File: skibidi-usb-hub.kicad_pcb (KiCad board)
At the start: 4 copper layers, 70 x 70 mm, 99 parts, among them SW1 B3U-1100PM, SW2 B3U-1100PM, T1 H1102NLT_C20623173, T2 H1102NLT_C20623173, U1 CH334F_C5187527, U10 PJ-320A-4P DIP, U2 CH217K, U3 GT-USB-7010ASV, U4 GT-USB-7010ASV, U5 RTL8152B-VB-CG, U6 GT-USB-7010ASV, U7 RTL8152B-VB-CG, U8 CH334F_C5187527, U9 HS-100B, X1 X322516MLB4SI, X2 X322516MLB4SI

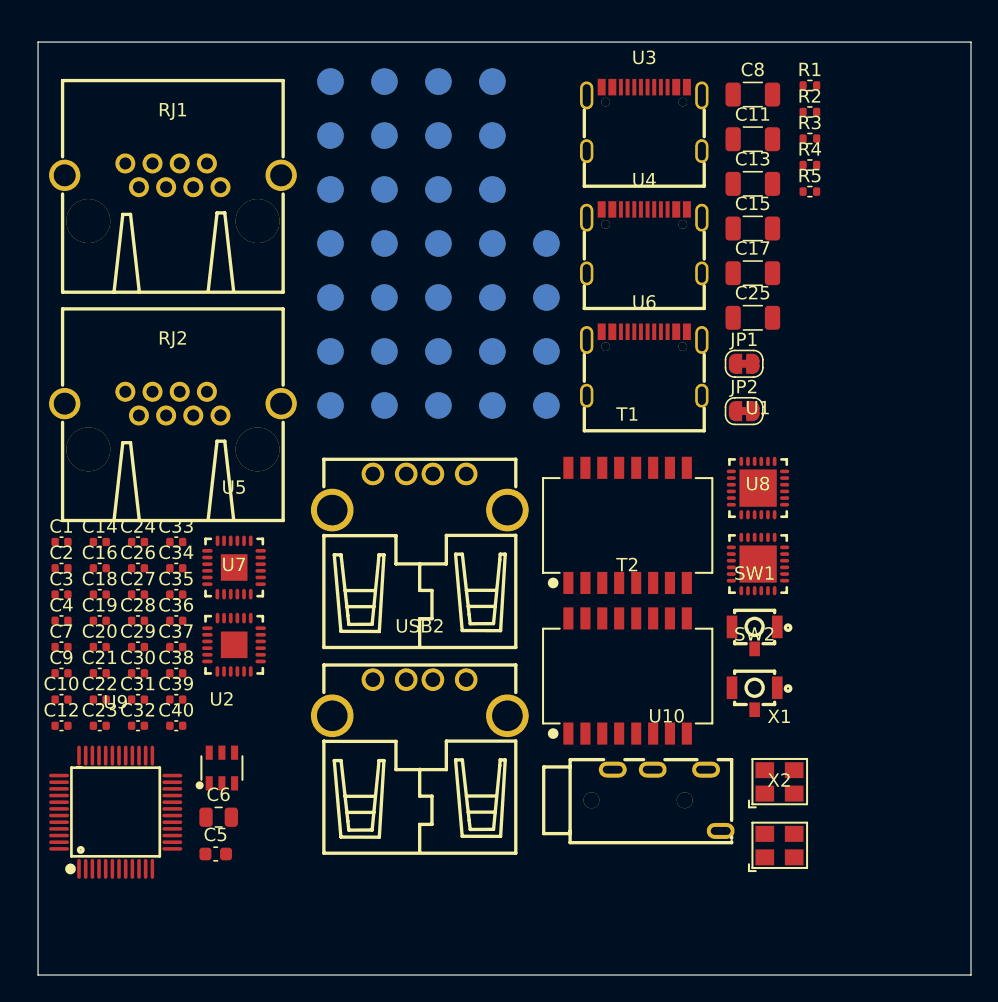
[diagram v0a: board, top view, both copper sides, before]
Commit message: PCB done!!!
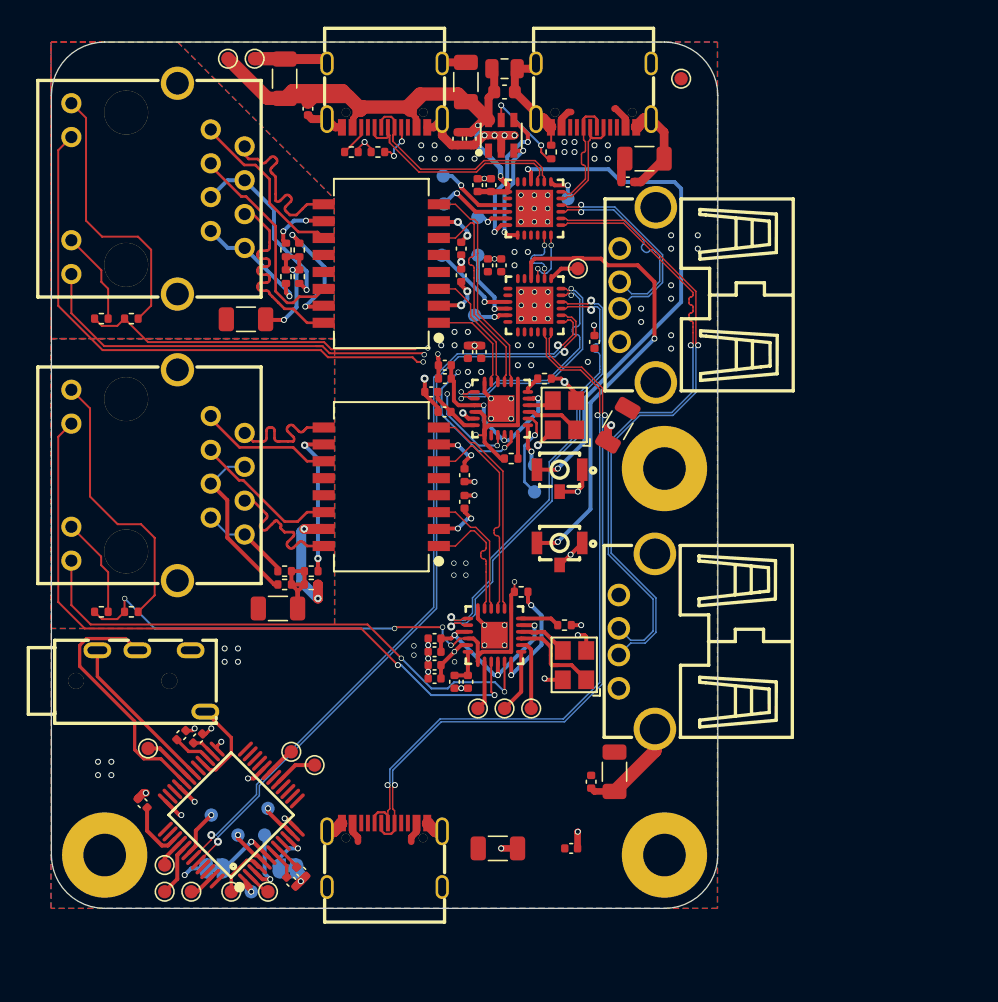
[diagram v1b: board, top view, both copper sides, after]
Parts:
- removed TP10, TP27, TP9: TestPoint, TestPoint:TestPoint_Pad_D2.0mm
- added C41: 1n, Capacitor_SMD:C_1206_3216Metric, F.Cu at (135.6, 80.8)
- added C42: 1n, Capacitor_SMD:C_1206_3216Metric, F.Cu at (138.0, 102.5)
- added H1: MountingHole, MountingHole:MountingHole_3.2mm_M3_Pad, F.Cu at (167.0, 121.0)
- added H2: MountingHole, MountingHole:MountingHole_3.2mm_M3_Pad, F.Cu at (167.0, 92.0)
- added H3: MountingHole, MountingHole:MountingHole_3.2mm_M3_Pad, F.Cu at (125.0, 121.0)
- added R10: 75, Resistor_SMD:R_0402_1005Metric, F.Cu at (139.6, 77.6)
- added R11: 75, Resistor_SMD:R_0402_1005Metric, F.Cu at (138.6, 77.6)
- added R12: 75, Resistor_SMD:R_0402_1005Metric, F.Cu at (140.5, 100.7)
- added R13: 75, Resistor_SMD:R_0402_1005Metric, F.Cu at (140.5, 99.7)
- added R14: 75, Resistor_SMD:R_0402_1005Metric, F.Cu at (138.5, 100.7)
- added R15: 75, Resistor_SMD:R_0402_1005Metric, F.Cu at (138.5, 99.7)
- added R16: 470, Resistor_SMD:R_0402_1005Metric, F.Cu at (127.0, 80.8)
- added R17: 470, Resistor_SMD:R_0402_1005Metric, F.Cu at (124.8, 80.8)
- added R18: 470, Resistor_SMD:R_0402_1005Metric, F.Cu at (127.0, 102.8)
- added R19: 470, Resistor_SMD:R_0402_1005Metric, F.Cu at (124.8, 102.8)
- added R6: 5.1k, Resistor_SMD:R_0402_1005Metric, F.Cu at (145.5, 68.2)
- added R7: 5.1k, Resistor_SMD:R_0402_1005Metric, F.Cu at (143.5, 68.2)
- added R8: 75, Resistor_SMD:R_0402_1005Metric, F.Cu at (139.6, 75.6)
- added R9: 75, Resistor_SMD:R_0402_1005Metric, F.Cu at (138.6, 75.6)
- JP1, JP2: moved to B.Cu
- RJ1, RJ2: value X12ADGWA3DY1027 -> R-RJ45S08P-C000; footprint easyeda2kicad:RJ45-TH_XKB_X12ADHWA3DY1027 -> easyeda2kicad:RJ45-TH_R-RJ45S08P-C000
- TP1, TP11, TP16, TP17, TP2, TP20, TP22, TP28, TP3, TP30, TP4, TP5, TP6, TP8: footprint TestPoint:TestPoint_Pad_D2.0mm -> TestPoint:TestPoint_Pad_D1.0mm
- TP12, TP13, TP14, TP15, TP18, TP19, TP21, TP23, TP24, TP25, TP26, TP33, TP35, TP36, TP7: footprint TestPoint:TestPoint_Pad_D2.0mm -> TestPoint:TestPoint_Pad_D1.0mm; moved to F.Cu
- moved TP14 63.0 mm to (129.5, 123.8)
- moved TP21 62.1 mm to (137.2, 123.8)
- moved C5 61.1 mm to (155.0, 63.8)
- moved C6 60.1 mm to (155.0, 62.0)
- moved TP20 58.4 mm to (136.0, 123.8)
- moved TP13 57.2 mm to (129.5, 121.8)
- moved JP2 52.5 mm to (133.2, 122.0)
- moved U2 51.9 mm to (154.8, 67.0)
- moved JP1 51.0 mm to (138.8, 122.0), turned to 180 degrees
- moved C16 49.1 mm to (164.2, 70.5)
- moved C10 48.0 mm to (140.2, 65.0), turned to -90 degrees
- moved C4 47.5 mm to (152.5, 67.2), turned to -90 degrees
- moved TP19 47.3 mm to (128.2, 113.0)
- moved TP11 45.7 mm to (135.0, 119.5)
- moved C3 45.3 mm to (151.5, 67.2), turned to -90 degrees
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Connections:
- C20 pad 1: +1V0 -> Net-(U5-AVDD10)
- C21 pad 1: +1V0 -> Net-(U5-AVDD10)
- C22 pad 1: +1V1 -> Net-(U5-DVDD10_UPS)
- C23 pad 1: +1V1 -> Net-(U5-DVDD10_UPS)
- C26 pad 1: +1V0 -> Net-(U7-AVDD10)
- C27 pad 1: +1V0 -> Net-(U7-AVDD10)
- C30 pad 1: +1V1 -> Net-(U7-DVDD10_UPS)
- C31 pad 1: +1V1 -> Net-(U7-DVDD10_UPS)
- C38 pad 1: Net-(C37-Pad1) -> Net-(C38-Pad1)
- C40 pad 1: Net-(C39-Pad1) -> Net-(C40-Pad1)
- R3 pad 1: +3.3V -> +3.3V2
- R4 pad 1: +3.3V -> +3.3V3
- RJ1 pad 1: Net-(RJ1-Pad1) -> /TDI0+
- RJ1 pad 10: /LED1 -> /LED0
- RJ1 pad 2: Net-(RJ1-Pad2) -> /TDI0-
- RJ1 pad 3: Net-(RJ1-Pad3) -> /TDI1+
- RJ1 pad 4: Net-(RJ1-Pad4) -> Net-(R10-Pad1)
- RJ1 pad 5: Net-(RJ1-Pad4) -> Net-(R10-Pad1)
- RJ1 pad 6: Net-(RJ1-Pad6) -> /TDI1-
- RJ1 pad 7: Net-(RJ1-Pad4) -> Net-(R11-Pad1)
- RJ1 pad 8: Net-(RJ1-Pad4) -> Net-(R11-Pad1)
- RJ1 pad 9: /LED0 -> Net-(RJ1-Y+)
- RJ2 pad 1: Net-(RJ2-Pad1) -> /TDI2+
- RJ2 pad 10: /LED3 -> /LED2
- RJ2 pad 2: Net-(RJ2-Pad2) -> /TDI2-
- RJ2 pad 3: Net-(RJ2-Pad3) -> /TDI3+
- RJ2 pad 4: Net-(RJ2-Pad4) -> Net-(R14-Pad1)
- RJ2 pad 5: Net-(RJ2-Pad4) -> Net-(R14-Pad1)
- RJ2 pad 6: Net-(RJ2-Pad6) -> /TDI3-
- RJ2 pad 7: Net-(RJ2-Pad4) -> Net-(R15-Pad1)
- RJ2 pad 8: Net-(RJ2-Pad4) -> Net-(R15-Pad1)
- RJ2 pad 9: /LED2 -> Net-(RJ2-Y+)
- T1 pad 1: /MDI0+ -> /MDI1-
- T1 pad 10: unconnected-(T1-Pad10) -> Net-(R9-Pad2)
- T1 pad 11: Net-(RJ1-Pad3) -> /TDI0+
- T1 pad 14: Net-(RJ1-Pad2) -> /TDI1+
- T1 pad 15: unconnected-(T1-Pad15) -> Net-(R8-Pad2)
- T1 pad 16: Net-(RJ1-Pad1) -> /TDI1-
- T1 pad 3: /MDI0- -> /MDI1+
- T1 pad 6: /MDI1+ -> /MDI0-
- T1 pad 7: Net-(C37-Pad1) -> Net-(C38-Pad1)
- T1 pad 8: /MDI1- -> /MDI0+
- T1 pad 9: Net-(RJ1-Pad6) -> /TDI0-
- T2 pad 1: /MDI2+ -> /MDI3-
- T2 pad 10: unconnected-(T2-Pad10) -> Net-(R13-Pad2)
- T2 pad 11: Net-(RJ2-Pad3) -> /TDI2+
- T2 pad 14: Net-(RJ2-Pad2) -> /TDI3+
- T2 pad 15: unconnected-(T2-Pad15) -> Net-(R12-Pad2)
- T2 pad 16: Net-(RJ2-Pad1) -> /TDI3-
- T2 pad 3: /MDI2- -> /MDI3+
- T2 pad 6: /MDI3+ -> /MDI2-
- T2 pad 7: Net-(C39-Pad1) -> Net-(C40-Pad1)
- T2 pad 8: /MDI3- -> /MDI2+
- T2 pad 9: Net-(RJ2-Pad6) -> /TDI2-
- U3 pad A5: unconnected-(U3-CC1-PadA5) -> Net-(U3-CC1)
- U3 pad B5: unconnected-(U3-CC2-PadB5) -> Net-(U3-CC2)
- U5 pad 1: +3.3V -> +3.3V2
- U5 pad 10: +3.3V -> +3.3V2
- U5 pad 12: +1V1 -> Net-(U5-DVDD10_UPS)
- U5 pad 13: +3.3V -> +3.3V2
- U5 pad 16: +1V0 -> Net-(U5-AVDD10)
- U5 pad 23: +1V0 -> Net-(U5-AVDD10)
- U5 pad 9: +1V0 -> Net-(U5-AVDD10)
- U7 pad 1: +3.3V -> +3.3V3
- U7 pad 10: +3.3V -> +3.3V3
- U7 pad 12: +1V1 -> Net-(U7-DVDD10_UPS)
- U7 pad 13: +3.3V -> +3.3V3
- U7 pad 16: +1V0 -> Net-(U7-AVDD10)
- U7 pad 23: +1V0 -> Net-(U7-AVDD10)
- U7 pad 9: +1V0 -> Net-(U7-AVDD10)
- U9 pad 13: Net-(U9-NC-Pad13) -> (no net)
- U9 pad 14: Net-(U9-NC-Pad13) -> (no net)
- U9 pad 15: Net-(U9-NC-Pad13) -> (no net)
- U9 pad 16: Net-(U9-NC-Pad13) -> (no net)
- U9 pad 18: Net-(U9-NC-Pad13) -> (no net)
- U9 pad 21: Net-(U9-NC-Pad13) -> (no net)
- U9 pad 22: Net-(U9-NC-Pad13) -> (no net)
- U9 pad 23: Net-(U9-NC-Pad13) -> (no net)
- U9 pad 24: Net-(U9-NC-Pad13) -> (no net)
- U9 pad 37: Net-(U9-NC-Pad13) -> (no net)
- U9 pad 38: Net-(U9-NC-Pad13) -> (no net)
- U9 pad 45: Net-(U9-NC-Pad13) -> (no net)
- U9 pad 46: Net-(U9-NC-Pad13) -> (no net)
- U9 pad 48: Net-(U9-NC-Pad13) -> (no net)
- U9 pad 9: Net-(U9-NC-Pad13) -> (no net)
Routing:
- net GND: track 0.00 -> 99.1 mm, vias 0 -> 64
- net VBUS: track 0.00 -> 61.4 mm, vias 0 -> 2
- net /D23+: track 0.00 -> 58.1 mm, vias 0 -> 2
- net /D23-: track 0.00 -> 57.6 mm, vias 0 -> 2
- net /D24+: track 0.00 -> 54.0 mm, vias 0 -> 2
- net /D24-: track 0.00 -> 54.0 mm, vias 0 -> 2
- net /LED0: track 0.00 -> 52.6 mm, vias 0 -> 3
- net /LED2: track 0.00 -> 52.0 mm, vias 0 -> 2
- net +3.3V2: track 0.00 -> 48.2 mm, vias 0 -> 2
- net /D3+: track 0.00 -> 47.1 mm, vias 0 -> 1
- net /D3-: track 0.00 -> 47.0 mm, vias 0 -> 1
- net /LED1: track 0.00 -> 45.1 mm, vias 0 -> 3
- net +3.3V3: track 0.00 -> 42.3 mm, vias 0 -> 5
- net /LED3: track 0.00 -> 41.2 mm, vias 0 -> 2
- net Net-(U1-~{RESET}/CDP): track 0.00 -> 39.6 mm, vias 0 -> 2
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- added copper zone on B.Cu, net +5V
- added copper zone on F.Cu, net +5V
- added copper zone on In1.Cu, net GND
- added copper zone on In2.Cu, net GND
- added copper zone on B.Cu, net GND2
- added copper zone on F.Cu, net GND2
- added copper zone on In1.Cu, net GND2
- added copper zone on In2.Cu, net GND2
- added copper zone on B.Cu, net GND3
- added copper zone on F.Cu, net GND3
- added copper zone on In1.Cu, net GND3
- added copper zone on In2.Cu, net GND3
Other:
- board size 70 x 70 mm -> 50 x 65 mm
- board text added: "@tobycm"
- board text added: "In one million year, people will read my message lol"
- board text added: "made by tobycm https://tobycm.dev"
- board text added: "made in"
- board text added: "shout out to 2026 penticton robotics, greyback construction, and scarlett steyn <3"
- board text added: "toby@vsus.app"
- board text added: "v1"
- board text added: "very cool usb hub"
